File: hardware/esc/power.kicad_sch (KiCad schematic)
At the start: 37 parts, among them U13 LMR51420YFDDCR, U14 LDL212PUR

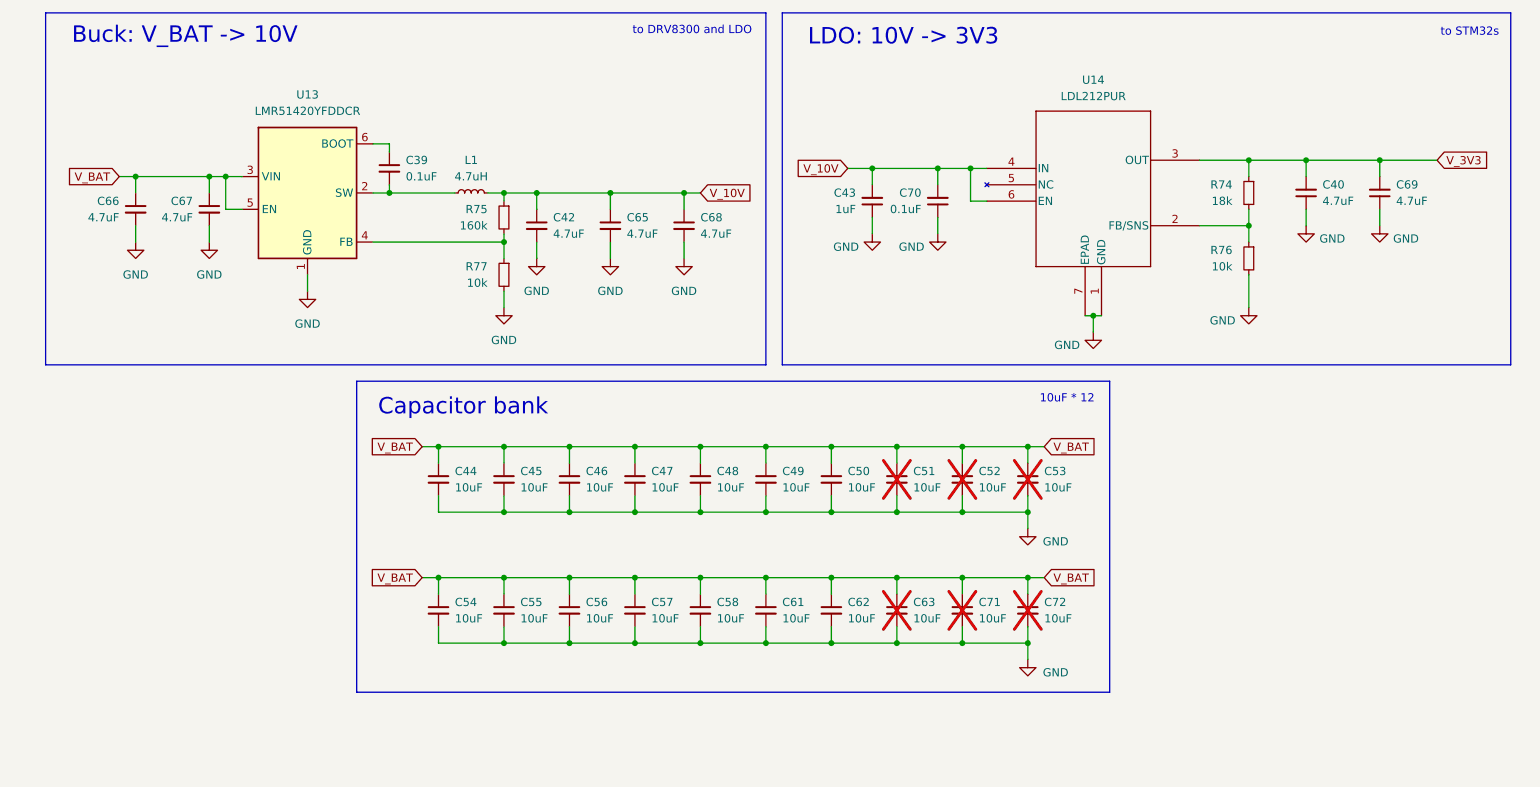
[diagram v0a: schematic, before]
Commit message: general: update ESC schem and README
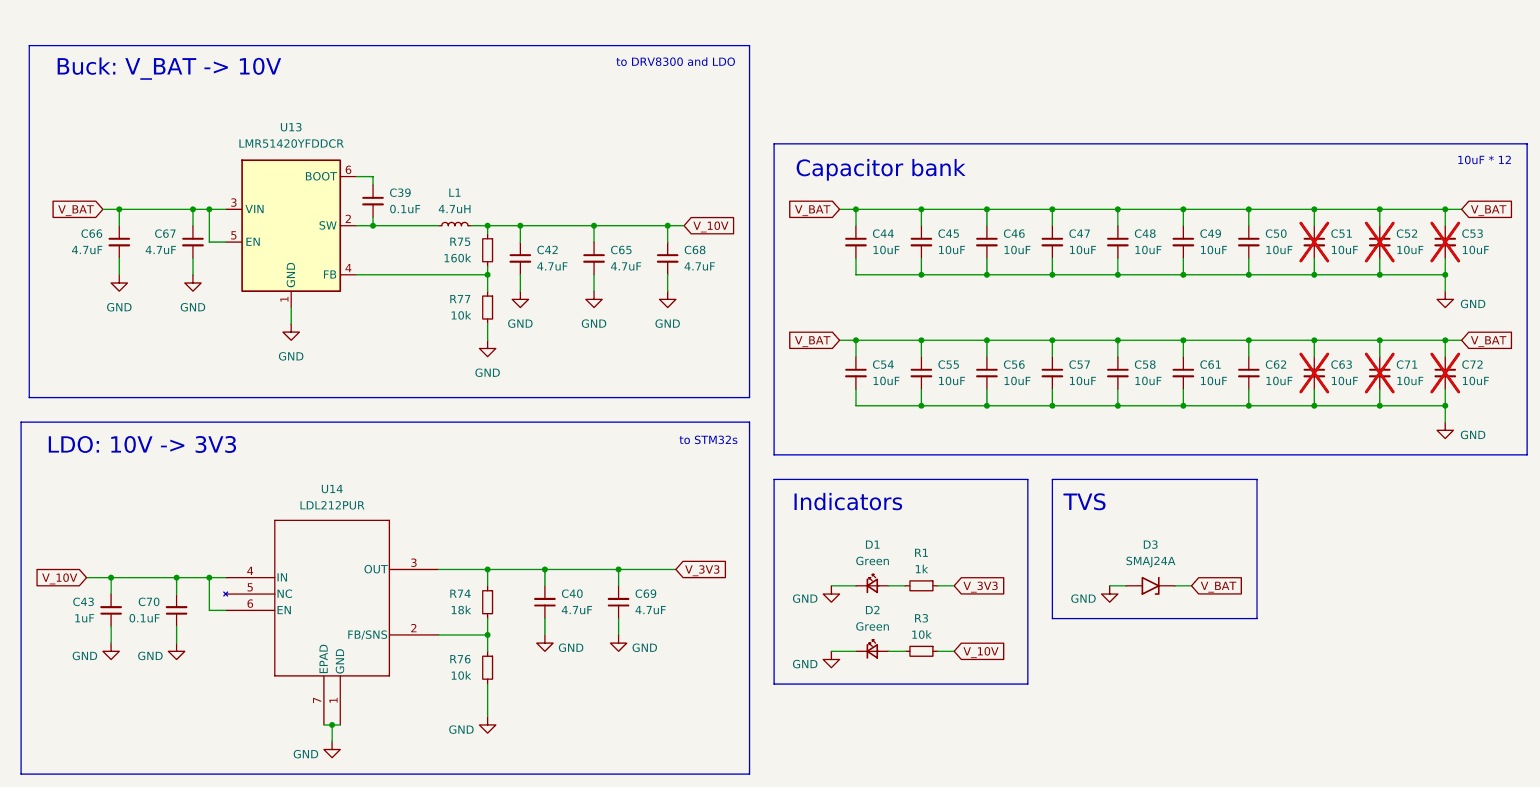
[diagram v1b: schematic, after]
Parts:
- added D1, D2: Green, LED_SMD:LED_0603_1608Metric, symbol Device:LED_Small
- added D3: SMAJ24A, Stratus:SMAJ20A, symbol Diode:SMAJ20A
- added R1: 1k, Stratus:R_0402, symbol Device:R_Small
- added R3: 10k, Stratus:R_0402, symbol Device:R_Small
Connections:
- net GND: now also D1.1 (K), D2.1 (K), D3.2 (A2)
- net V_10V: now also R3.1
- net V_3V3: now also R1.1
- net V_BAT: now also D3.1 (A1)
- new net: D2.2 (A), R3.2
- new net: D1.2 (A), R1.2
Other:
- note added: "Indicators"
- note added: "TVS"
- moved on the sheet: C39, C40, C42, C43, C44, C45, C46, C47, C48, C49, C50, C51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
